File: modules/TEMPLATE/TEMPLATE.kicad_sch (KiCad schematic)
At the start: 2 parts, among them J1 CardConnector

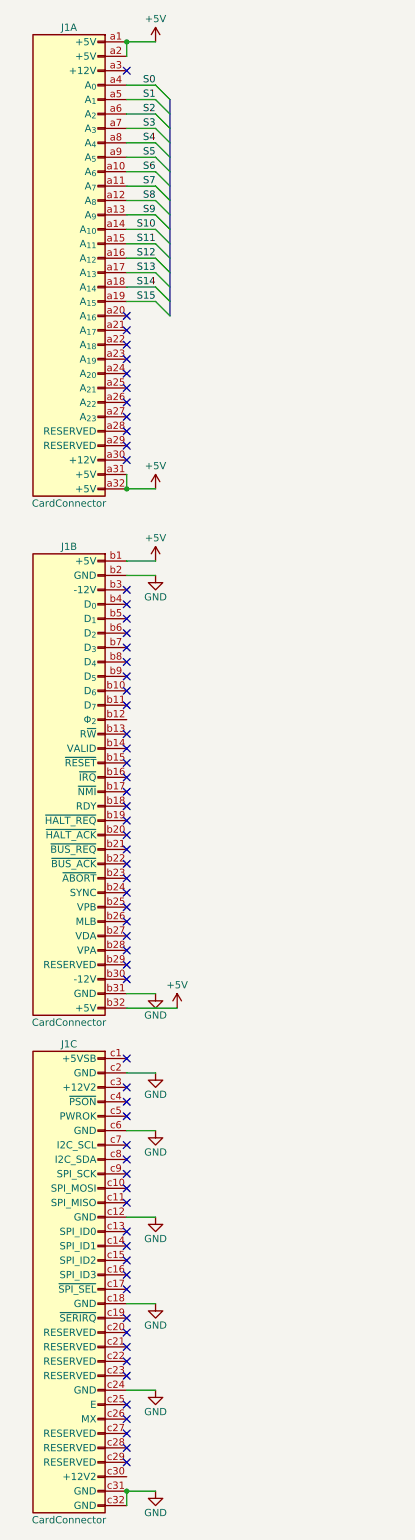
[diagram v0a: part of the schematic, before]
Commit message: numerous updates; documentation, ferruous, lightman, etc.
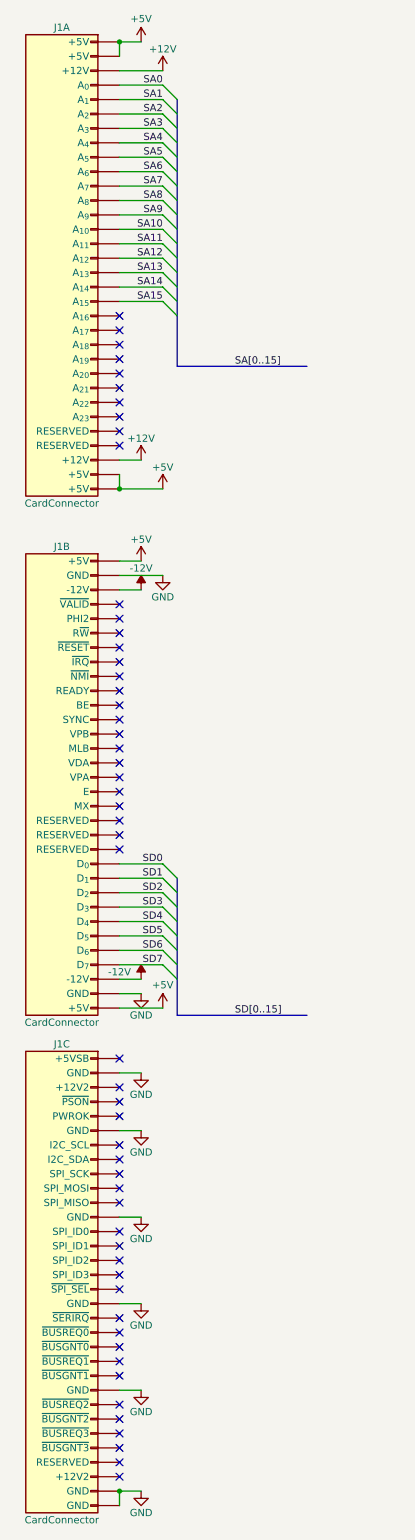
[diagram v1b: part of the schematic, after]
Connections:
- net SD0: now reaches J1.b22 (D_{0})
- net SD1: now reaches J1.b23 (D_{1})
- net SD2: now reaches J1.b24 (D_{2})
- net SD3: now reaches J1.b25 (D_{3})
- net SD4: now reaches J1.b26 (D_{4})
- net SD5: now reaches J1.b27 (D_{5})
- net SD6: now reaches J1.b28 (D_{6})
- net SD7: now reaches J1.b29 (D_{7})
- net -12V: now reaches J1.b3 (-12V)
- net -12V: now also J1.b30 (-12V)
- net +12V: now reaches J1.a3 (+12V)
- net +12V: now also J1.a30 (+12V)
- net S0 renamed SA0
- net S1 renamed SA1
- net S10 renamed SA10
- net S11 renamed SA11
- net S12 renamed SA12
- net S13 renamed SA13
- net S14 renamed SA14
- net S15 renamed SA15
- net S2 renamed SA2
- net S3 renamed SA3
- net S4 renamed SA4
- net S5 renamed SA5
- net S6 renamed SA6
- net S7 renamed SA7
- net S8 renamed SA8
- net S9 renamed SA9
- no-connect marks 63 -> 53

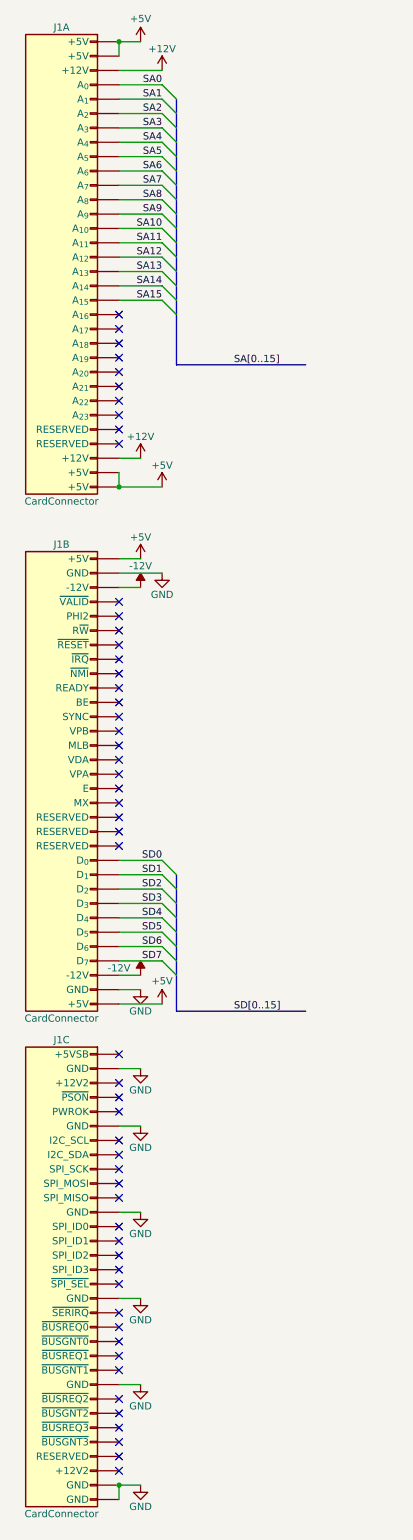
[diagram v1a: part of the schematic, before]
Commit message: added termination XXX card
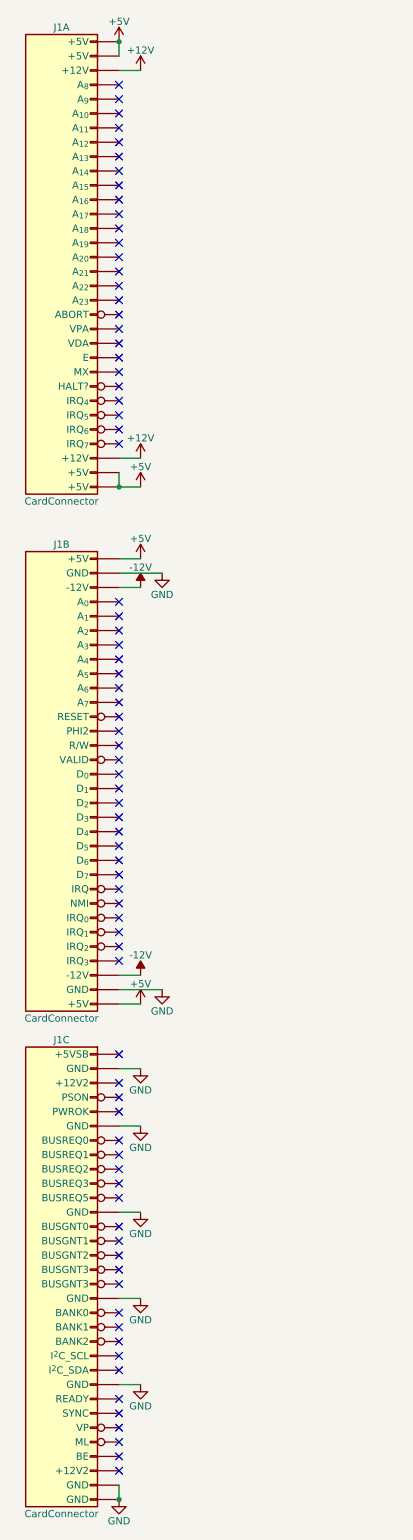
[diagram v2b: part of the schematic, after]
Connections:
- net SA0: no longer names the net of J1.a4 (A_{8})
- net SA1: no longer names the net of J1.a5 (A_{9})
- net SA10: no longer names the net of J1.a14 (A_{18})
- net SA11: no longer names the net of J1.a15 (A_{19})
- net SA12: no longer names the net of J1.a16 (A_{20})
- net SA13: no longer names the net of J1.a17 (A_{21})
- net SA14: no longer names the net of J1.a18 (A_{22})
- net SA15: no longer names the net of J1.a19 (A_{23})
- net SA2: no longer names the net of J1.a6 (A_{10})
- net SA3: no longer names the net of J1.a7 (A_{11})
- net SA4: no longer names the net of J1.a8 (A_{12})
- net SA5: no longer names the net of J1.a9 (A_{13})
- net SA6: no longer names the net of J1.a10 (A_{14})
- net SA7: no longer names the net of J1.a11 (A_{15})
- net SA8: no longer names the net of J1.a12 (A_{16})
- net SA9: no longer names the net of J1.a13 (A_{17})
- net SD0: no longer names the net of J1.b22 (D_{6})
- net SD1: no longer names the net of J1.b23 (D_{7})
- net SD2: no longer names the net of J1.b24 (IRQ)
- net SD3: no longer names the net of J1.b25 (NMI)
- net SD4: no longer names the net of J1.b26 (IRQ_{0})
- net SD5: no longer names the net of J1.b27 (IRQ_{1})
- net SD6: no longer names the net of J1.b28 (IRQ_{2})
- net SD7: no longer names the net of J1.b29 (IRQ_{3})
- no-connect marks 53 -> 77

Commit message: added 9V power supply
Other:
- company: THE HOUSE OF GALAHAD -> ${COMPANY_NAME}
- title: TITLE -> ${MODULE_NAME}
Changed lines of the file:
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@@
 	(paper "A3")
 	(title_block
-		(title "TITLE")
+		(title "${MODULE_NAME}")
 		(rev "A")
-		(company "THE HOUSE OF GALAHAD")
-		(comment 1 "IMNOTWOPR")
-		(comment 2 "CARD TEMPLATE")
-		(comment 3 "75-1000-01")
+		(company "${COMPANY_NAME}")
+		(comment 1 "${PROJECT_NAME}")
+		(comment 2 "${MODULE_DESCRIPTION}")
+		(comment 3 "${PART_NUMBER}")
 	)
 	(junction
